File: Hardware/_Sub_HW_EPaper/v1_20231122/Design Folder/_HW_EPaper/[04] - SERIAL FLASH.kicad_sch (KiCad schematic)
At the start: 5 parts, among them U401 W25Q64JVSSIQ

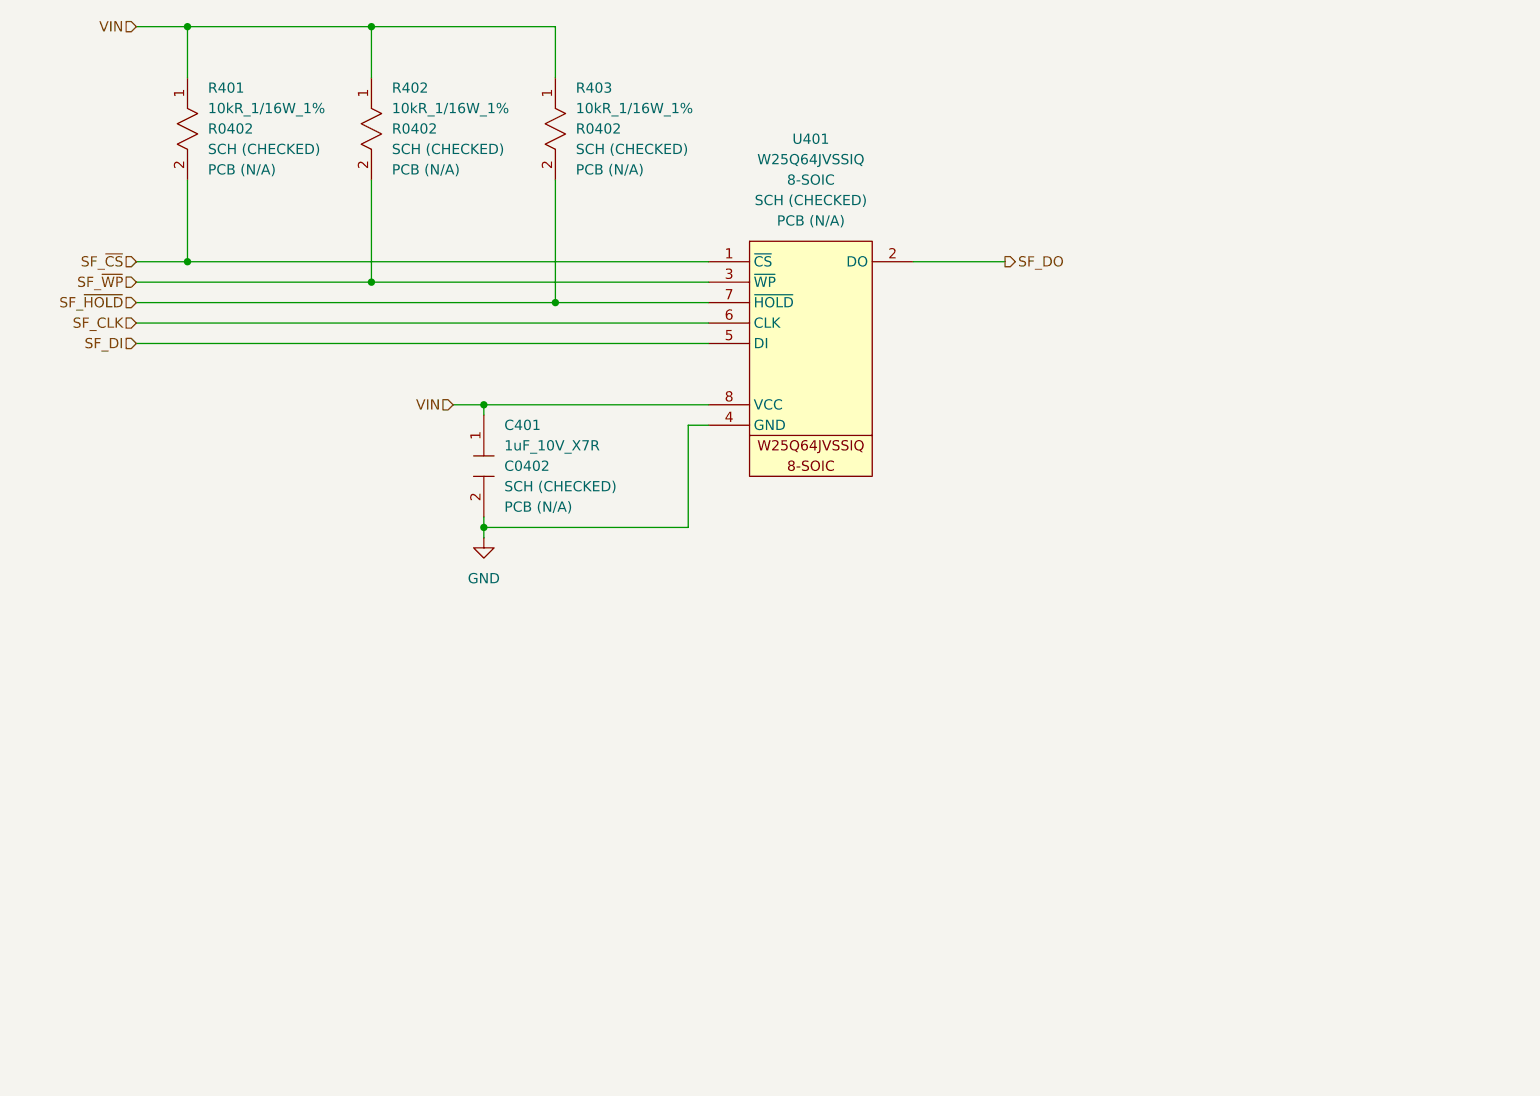
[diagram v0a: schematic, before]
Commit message: Updating file templates and structures...
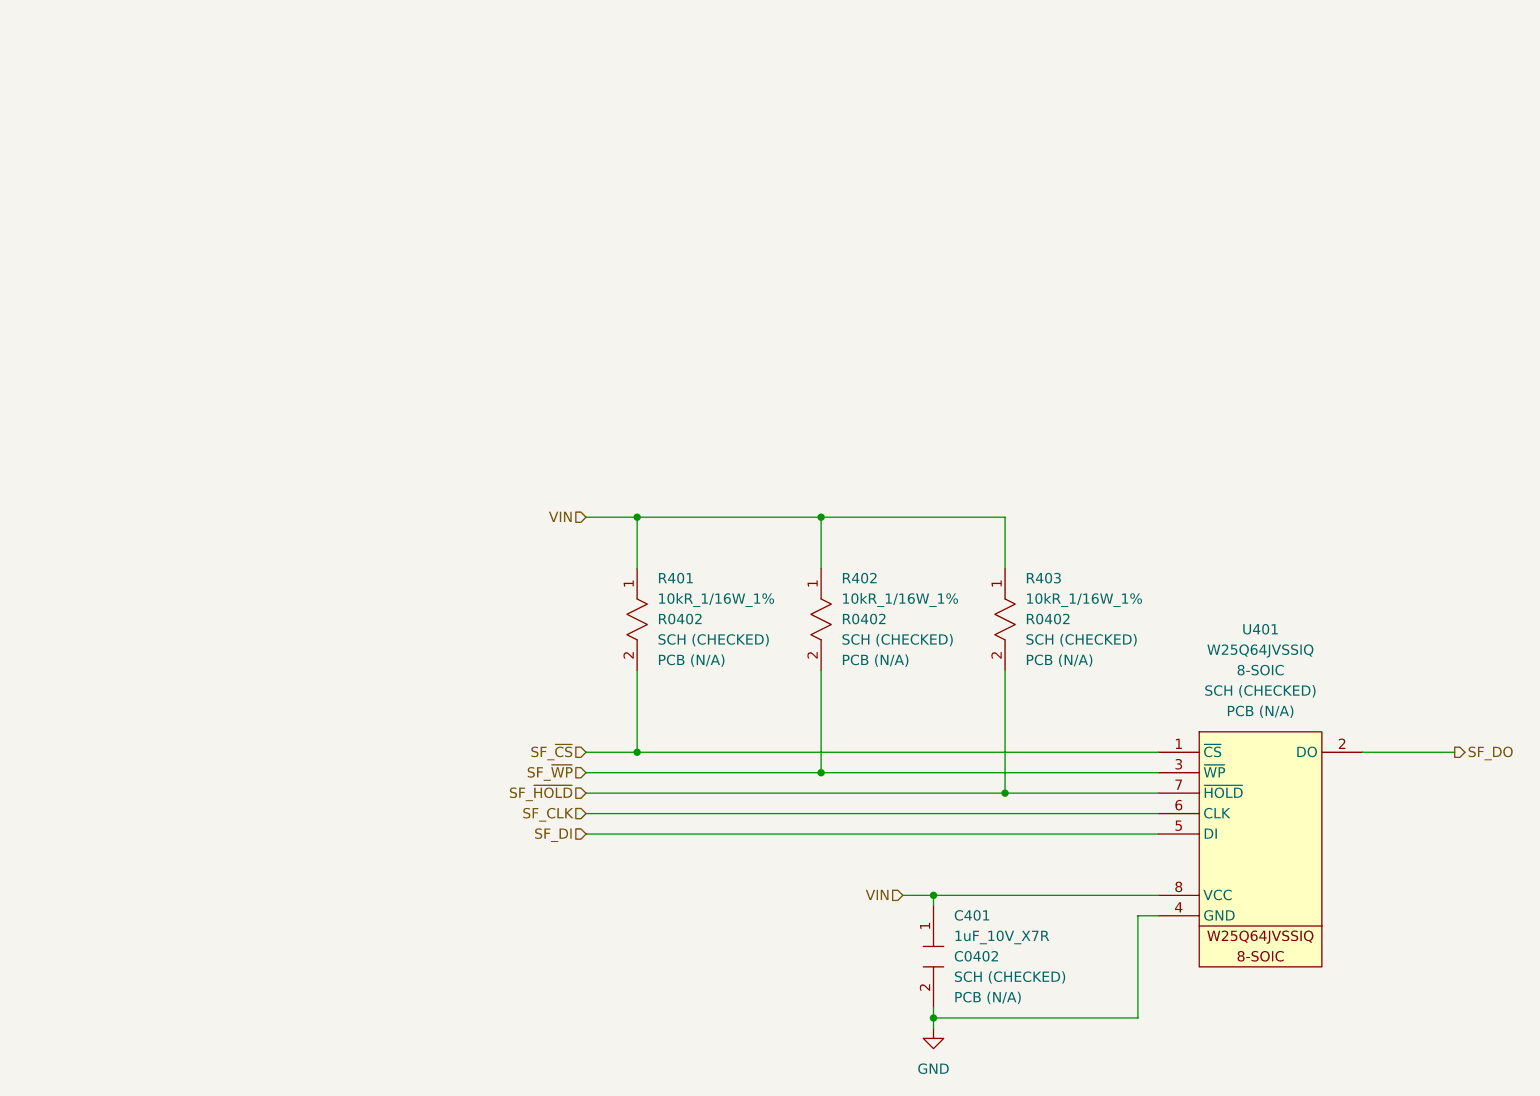
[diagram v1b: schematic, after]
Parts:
- C401: Manufacturer (none) -> Murata Electronics; Part Number GRM155Z71A105KE01D -> (none); Part Number (Manufacturer) (none) -> GRM155Z71A105KE01D; Part Number (Vendor) (none) -> 490-GRM155Z71A105KE01DTR-ND; Vendor (none) -> Digikey
- R401, R402, R403: Manufacturer (none) -> Bourns Inc.; Part Number CR0402-FX-1002GLF -> (none); Part Number (Manufacturer) (none) -> CR0402-FX-1002GLF; Part Number (Vendor) (none) -> CR0402-FX-1002GLFTR-ND; Vendor (none) -> Digikey
- U401: Manufacturer (none) -> Winbond Electronics; Part Number W25Q64JVSSIQ -> (none); Part Number (Manufacturer) (none) -> W25Q64JVSSIQ; Part Number (Vendor) (none) -> W25Q64JVSSIQ-ND; Vendor (none) -> Digikey
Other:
- moved on the sheet: C401, R401, R402, R403, U401
